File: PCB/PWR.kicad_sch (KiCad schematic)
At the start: 71 parts, among them U201 STC3115IQT, U202 BQ25606RGER, U203 STPMIC1APQR

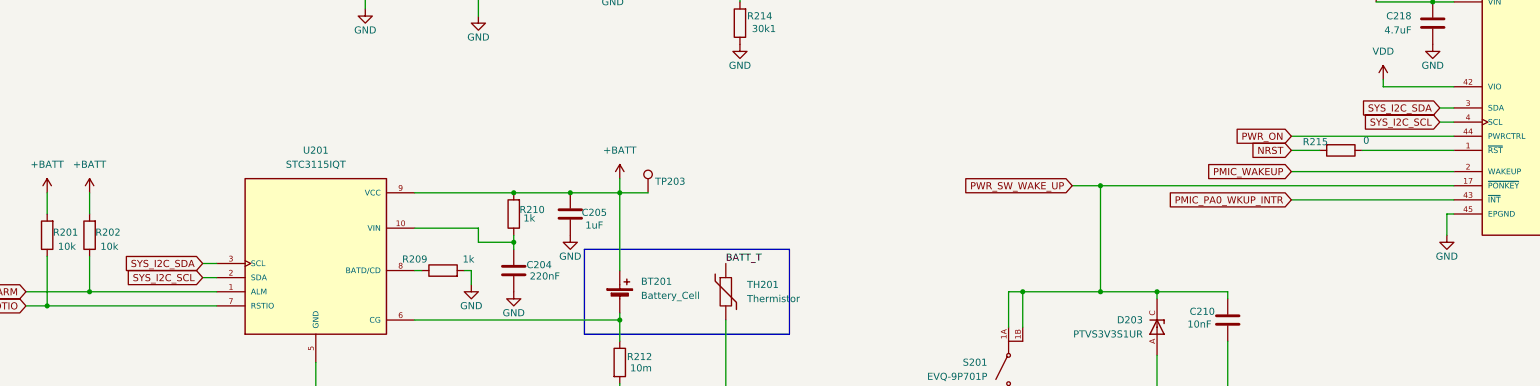
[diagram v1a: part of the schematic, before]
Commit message: pcb_update
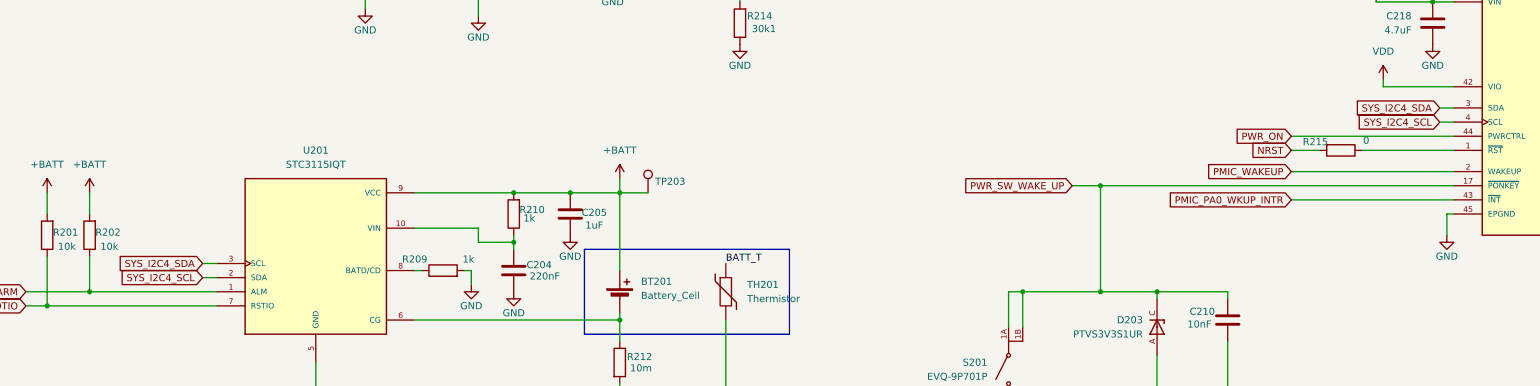
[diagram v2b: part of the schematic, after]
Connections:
- net SYS_I2C_SCL renamed SYS_I2C4_SCL
- net SYS_I2C_SDA renamed SYS_I2C4_SDA
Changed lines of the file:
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@@
 		)
 	)
-	(global_label "SYS_I2C_SCL"
+	(global_label "SYS_I2C4_SCL"
 		(shape input)
 		(at 307.34 217.17 180)
@@
 		)
 		(property "Intersheetrefs" "${INTERSHEET_REFS}"
-			(at 292.3201 217.17 0)
+			(at 291.1106 217.17 0)
 			(effects
 				(font
@@
 		)
 	)
-	(global_label "SYS_I2C_SDA"
+	(global_label "SYS_I2C4_SDA"
 		(shape input)
 		(at 85.09 242.57 180)
@@
 		)
 		(property "Intersheetrefs" "${INTERSHEET_REFS}"
-			(at 70.0096 242.57 0)
+			(at 68.8001 242.57 0)
 			(effects
 				(font
@@
 		)
 	)
-	(global_label "SYS_I2C_SCL"
+	(global_label "SYS_I2C4_SCL"
 		(shape input)
 		(at 85.09 245.11 180)
@@
 		)
 		(property "Intersheetrefs" "${INTERSHEET_REFS}"
-			(at 70.0701 245.11 0)
+			(at 68.8606 245.11 0)
 			(effects
 				(font
@@
 		)
 	)
-	(global_label "SYS_I2C_SDA"
+	(global_label "SYS_I2C4_SDA"
 		(shape input)
 		(at 307.34 214.63 180)
@@
 		)
 		(property "Intersheetrefs" "${INTERSHEET_REFS}"
-			(at 292.2596 214.63 0)
+			(at 291.0501 214.63 0)
 			(effects
 				(font
